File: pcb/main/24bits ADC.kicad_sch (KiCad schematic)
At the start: 8 parts, among them J8 SJ, U6 HX711

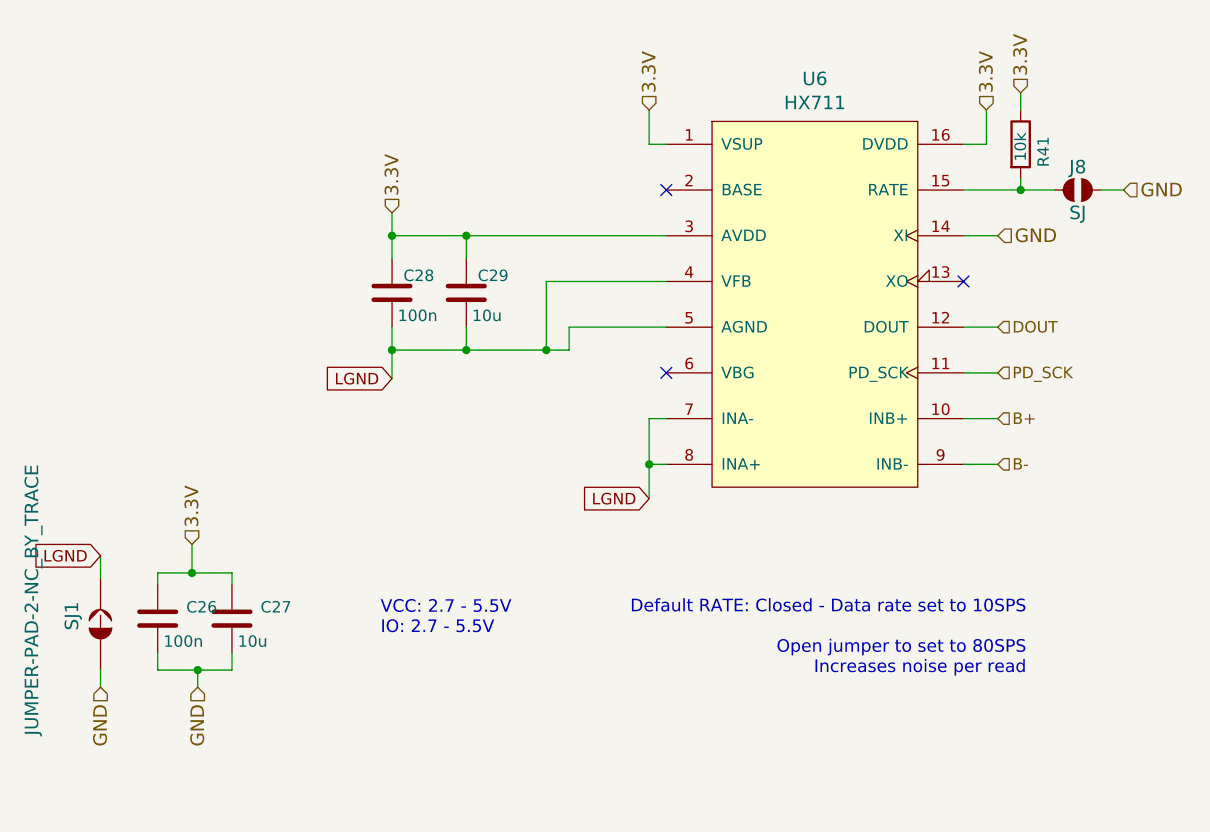
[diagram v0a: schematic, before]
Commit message: feat: updated BOM information
Some components are still without MNF and Seller information
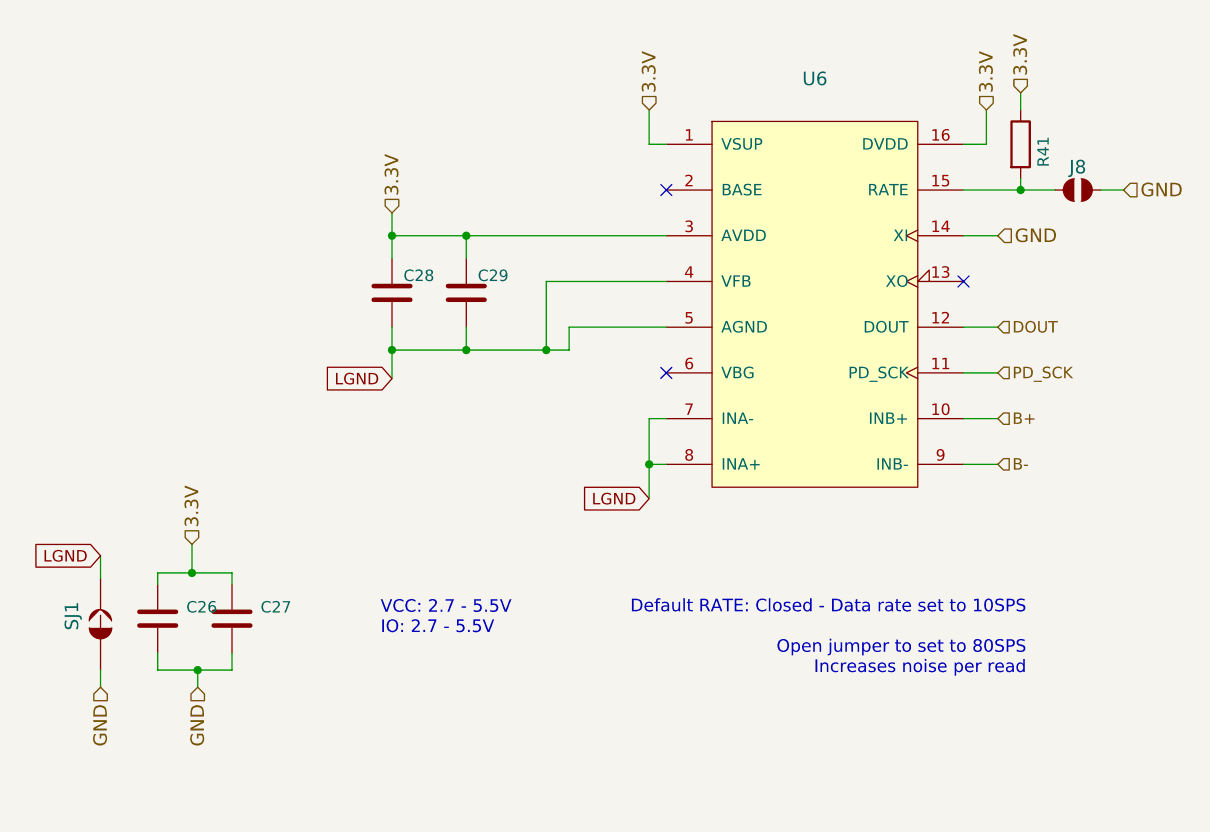
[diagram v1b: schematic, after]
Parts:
- C26, C28: value 100n -> (none); footprint Capacitor_SMD:C_0805_2012Metric_Pad1.18x1.45mm_HandSolder -> (none)
- C27, C29: value 10u -> (none); footprint Capacitor_SMD:C_0805_2012Metric_Pad1.18x1.45mm_HandSolder -> (none)
- J8: value SJ -> (none); footprint Jumper:SolderJumper-2_P1.3mm_Open_RoundedPad1.0x1.5mm -> (none)
- R41: value 10k -> (none); footprint Resistor_SMD:R_0805_2012Metric_Pad1.20x1.40mm_HandSolder -> (none)
- SJ1: value JUMPER-PAD-2-NC_BY_TRACE -> (none); footprint Jumper:SolderJumper-2_P1.3mm_Open_RoundedPad1.0x1.5mm -> (none)
- U6: value HX711 -> (none); footprint Package_SO:SOIC-16_3.9x9.9mm_P1.27mm -> (none)
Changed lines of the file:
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@@
       (effects (font (size 1.4986 1.4986)) (justify right))
     )
-    (property "Value" "JUMPER-PAD-2-NC_BY_TRACE" (id 1) (at 82.55 106.68 0)
+    (property "Value" "" (id 1) (at 82.55 106.68 0)
       (effects (font (size 1.4986 1.4986)) (justify right))
     )
-    (property "Footprint" "Jumper:SolderJumper-2_P1.3mm_Open_RoundedPad1.0x1.5mm" (id 2) (at 90.17 124.46 0)
+    (property "Footprint" "" (id 2) (at 90.17 124.46 0)
       (effects (font (size 1.27 1.27)) hide)
     )
@@
       (effects (font (size 1.27 1.27)) (justify left))
     )
-    (property "Value" "100n" (id 1) (at 97.155 126.365 0)
+    (property "Value" "" (id 1) (at 97.155 126.365 0)
       (effects (font (size 1.27 1.27)) (justify left))
     )
-    (property "Footprint" "Capacitor_SMD:C_0805_2012Metric_Pad1.18x1.45mm_HandSolder" (id 2) (at 97.4852 127.635 0)
+    (property "Footprint" "" (id 2) (at 97.4852 127.635 0)
       (effects (font (size 1.27 1.27)) hide)
     )
@@
       (effects (font (size 1.27 1.27)) (justify left))
     )
-    (property "Value" "10u" (id 1) (at 105.41 126.365 0)
+    (property "Value" "" (id 1) (at 105.41 126.365 0)
       (effects (font (size 1.27 1.27)) (justify left))
     )
-    (property "Footprint" "Capacitor_SMD:C_0805_2012Metric_Pad1.18x1.45mm_HandSolder" (id 2) (at 105.7402 127.635 0)
+    (property "Footprint" "" (id 2) (at 105.7402 127.635 0)
       (effects (font (size 1.27 1.27)) hide)
     )
@@
       (effects (font (size 1.27 1.27)) (justify left))
     )
-    (property "Value" "100n" (id 1) (at 123.19 90.17 0)
+    (property "Value" "" (id 1) (at 123.19 90.17 0)
       (effects (font (size 1.27 1.27)) (justify left))
     )
-    (property "Footprint" "Capacitor_SMD:C_0805_2012Metric_Pad1.18x1.45mm_HandSolder" (id 2) (at 123.5202 91.44 0)
+    (property "Footprint" "" (id 2) (at 123.5202 91.44 0)
       (effects (font (size 1.27 1.27)) hide)
     )
@@
       (effects (font (size 1.27 1.27)) (justify left))
     )
-    (property "Value" "10u" (id 1) (at 131.445 90.17 0)
+    (property "Value" "" (id 1) (at 131.445 90.17 0)
       (effects (font (size 1.27 1.27)) (justify left))
     )
-    (property "Footprint" "Capacitor_SMD:C_0805_2012Metric_Pad1.18x1.45mm_HandSolder" (id 2) (at 131.7752 91.44 0)
+    (property "Footprint" "" (id 2) (at 131.7752 91.44 0)
       (effects (font (size 1.27 1.27)) hide)
     )
@@
       (effects (font (size 1.4986 1.4986)))
     )
-    (property "Value" "SJ" (id 1) (at 198.755 78.74 0)
+    (property "Value" "" (id 1) (at 198.755 78.74 0)
       (effects (font (size 1.4986 1.4986)))
     )
-    (property "Footprint" "Jumper:SolderJumper-2_P1.3mm_Open_RoundedPad1.0x1.5mm" (id 2) (at 198.755 76.2 0)
+    (property "Footprint" "" (id 2) (at 198.755 76.2 0)
       (effects (font (size 1.27 1.27)) hide)
     )
@@
       (effects (font (size 1.27 1.27)) (justify left))
     )
-    (property "Value" "10k" (id 1) (at 192.405 73.025 90)
+    (property "Value" "" (id 1) (at 192.405 73.025 90)
       (effects (font (size 1.27 1.27)) (justify left))
     )
-    (property "Footprint" "Resistor_SMD:R_0805_2012Metric_Pad1.20x1.40mm_HandSolder" (id 2) (at 190.627 71.12 90)
+    (property "Footprint" "" (id 2) (at 190.627 71.12 90)
       (effects (font (size 1.27 1.27)) hide)
     )
@@
       (effects (font (size 1.4986 1.4986)))
     )
-    (property "Value" "HX711" (id 1) (at 169.545 66.5226 0)
+    (property "Value" "" (id 1) (at 169.545 66.5226 0)
       (effects (font (size 1.4986 1.4986)))
     )
-    (property "Footprint" "Package_SO:SOIC-16_3.9x9.9mm_P1.27mm" (id 2) (at 170.815 115.57 0)
+    (property "Footprint" "" (id 2) (at 170.815 115.57 0)
       (effects (font (size 1.27 1.27)) hide)
     )
